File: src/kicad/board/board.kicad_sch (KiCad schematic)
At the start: 19 parts, among them J1 USB_C_Receptacle_USB2.0, J2 Conn_01x06, J3 Micro_SD_Card_Det, J4 Conn_01x06_Male, J5 Conn_01x06_Male, U1 SRV05-4

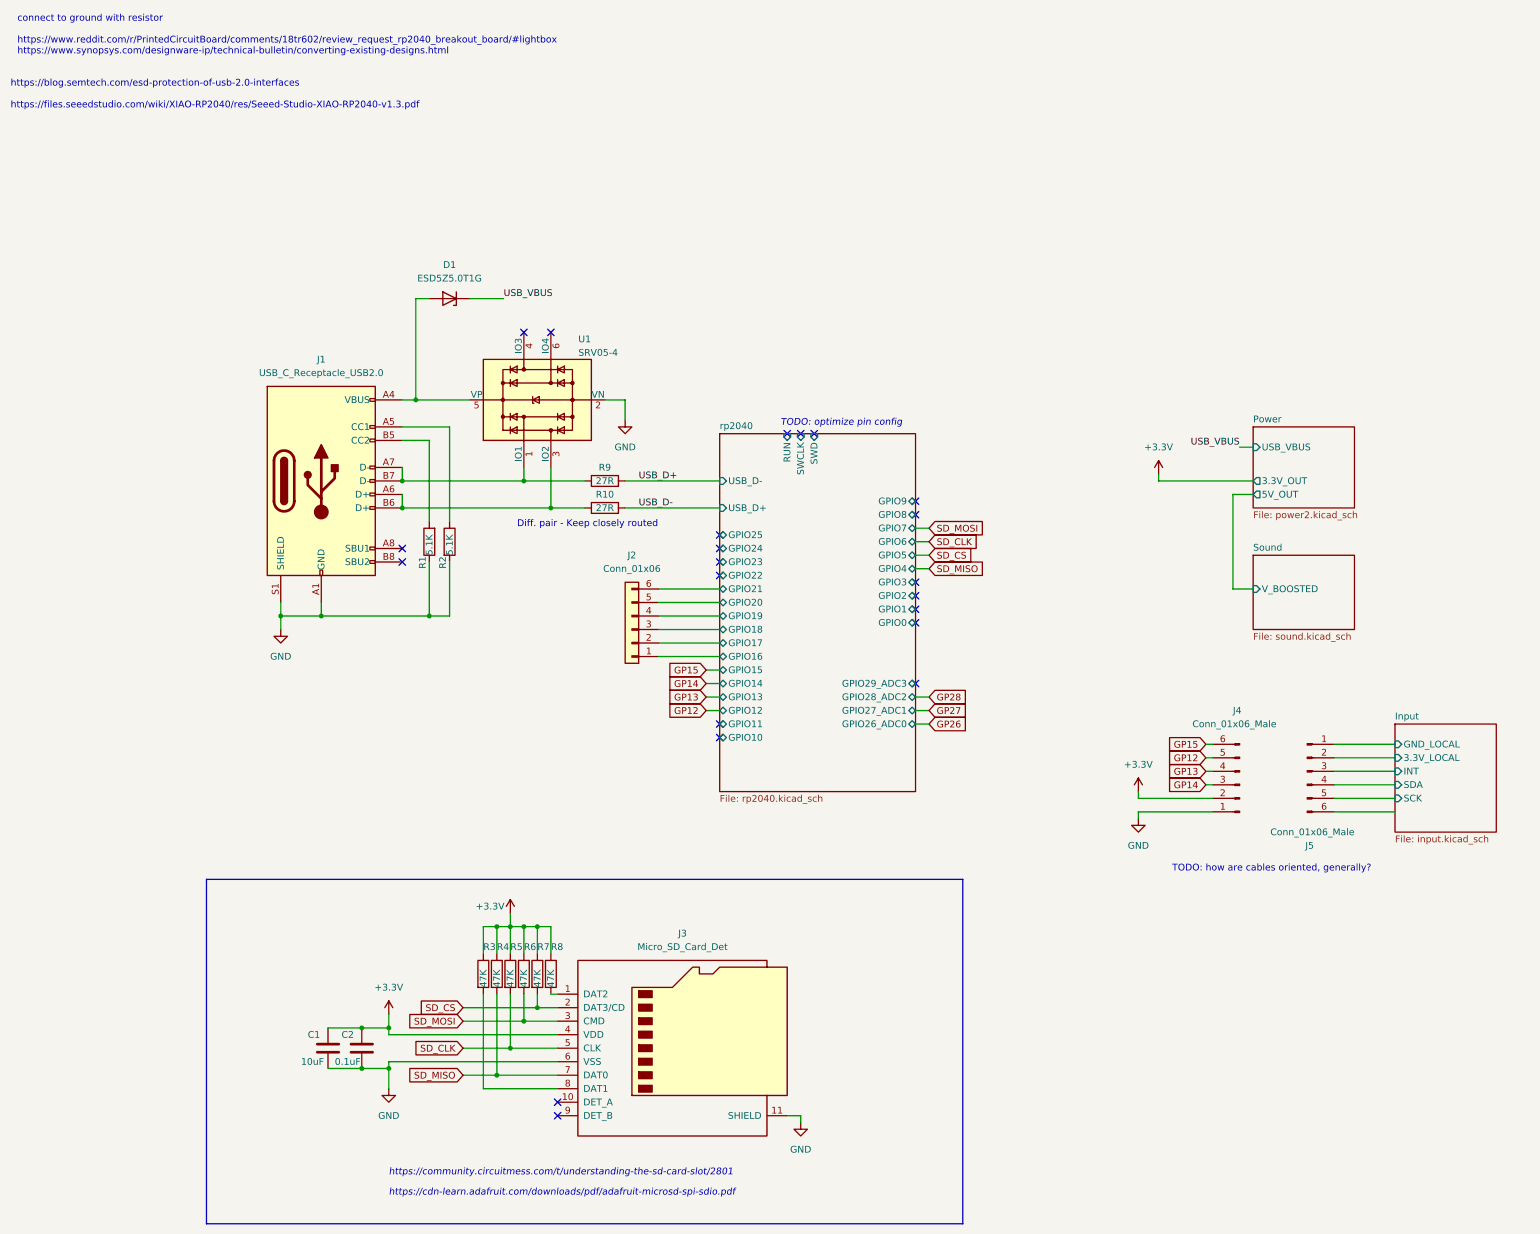
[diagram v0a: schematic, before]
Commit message: update
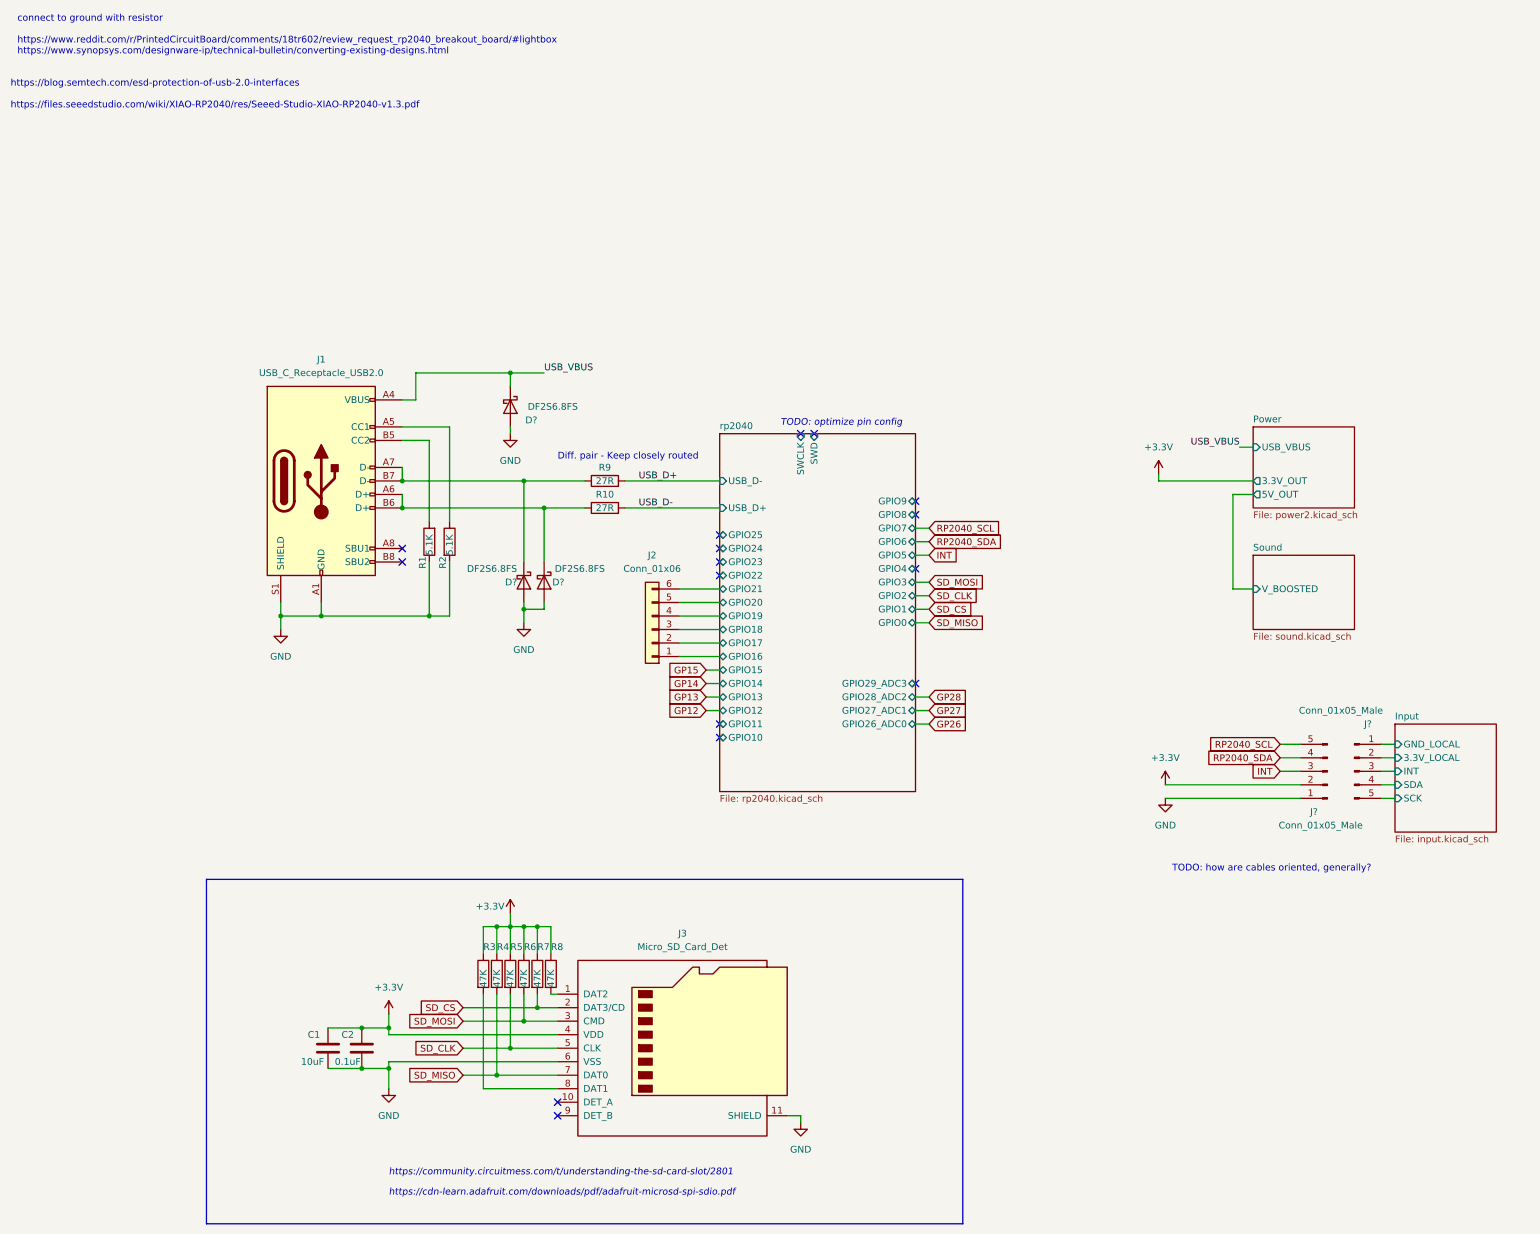
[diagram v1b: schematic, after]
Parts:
- removed D1: ESD5Z5.0T1G, Diode_SMD:D_SOD-523, symbol Diode:ESD5Zxx
- removed J4, J5: Conn_01x06_Male, Connector_JST:JST_PH_B6B-PH-SM4-TB_1x06-1MP_P2.00mm_Vertical, symbol Connector:Conn_01x06_Male
- removed U1: SRV05-4, Package_TO_SOT_SMD:SOT-23-6, symbol Power_Protection:SRV05-4
- added D? (x3): DF2S6.8FS, Diode_SMD:D_SOD-923, symbol Device:D_Schottky
- added J? (x2): Conn_01x05_Male, Connector_JST:JST_PH_B5B-PH-SM4-TB_1x05-1MP_P2.00mm_Vertical, symbol Connector:Conn_01x05_Male
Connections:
- net +3.3V: now also J?.2 (Pin_2)
- net GND: now also D?.2 (A), D?.2 (A), D?.2 (A), J?.1 (Pin_1)
- net Input/3.3V_LOCAL: now also J?.2 (Pin_2)
- net Input/GND_LOCAL: now also J?.1 (Pin_1)
- net Input/INT: now also J?.3 (Pin_3)
- net Input/SCK: now also J?.5 (Pin_5)
- net Input/SDA: now also J?.4 (Pin_4)
- net USB_VBUS: now also J1.A4 (VBUS), J1.A9 (VBUS), J1.B4 (VBUS), J1.B9 (VBUS), D?.1 (K)
- net at J1.A6 (D+), J1.B6 (D+), R10.1: now also D?.1 (K)
- net at J1.A7 (D-), J1.B7 (D-), R9.1: now also D?.1 (K)
- new net INT: J?.3 (Pin_3)
- new net RP2040_SCL: J?.5 (Pin_5)
- new net RP2040_SDA: J?.4 (Pin_4)
- no-connect marks 22 -> 16
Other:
- sheet rp2040 ports: added none; removed RUN
- moved on the sheet: J2
